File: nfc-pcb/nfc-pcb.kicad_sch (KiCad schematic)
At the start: 1 part, among them U1 NT3H1101W0FHKH

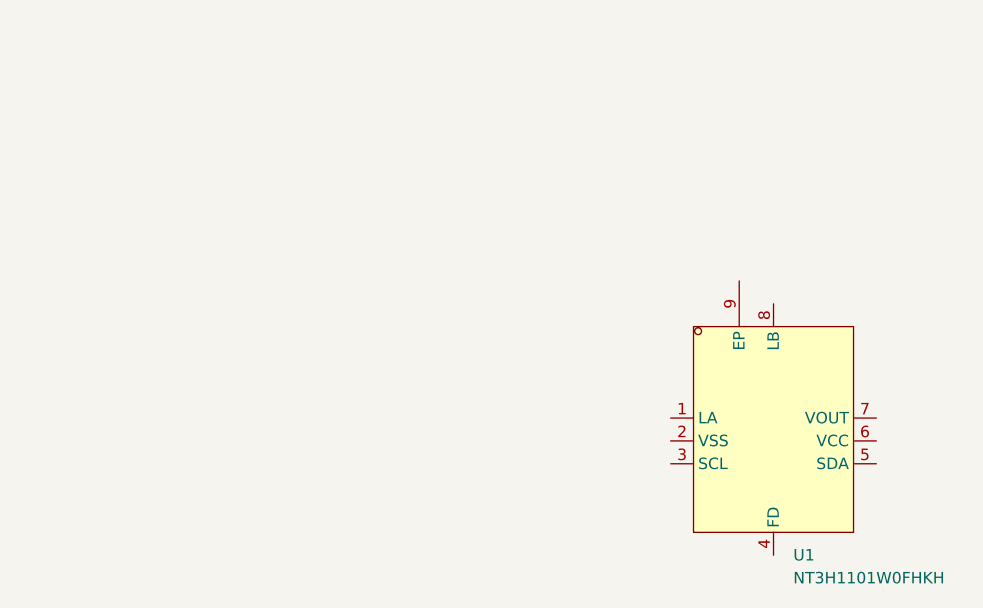
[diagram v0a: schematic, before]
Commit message: update
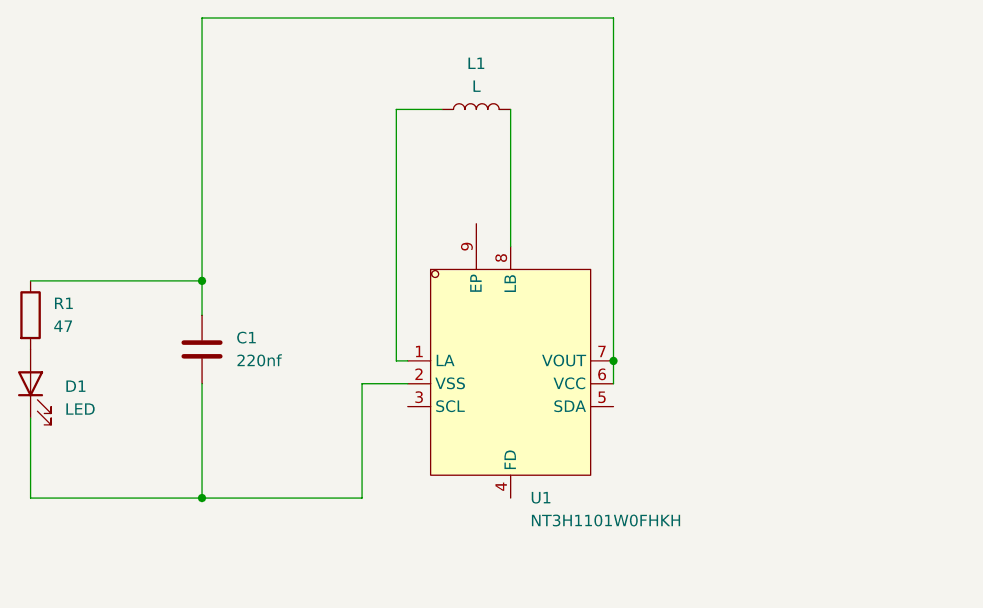
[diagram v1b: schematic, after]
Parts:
- added C1: 220nf, symbol Device:C
- added D1: LED, symbol Device:LED
- added L1: L, symbol Device:L
- added R1: 47, symbol Device:R
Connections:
- net at U1.1 (LA): now also L1.1
- net at U1.2 (VSS): now also C1.2, D1.1 (K)
- net at U1.6 (VCC): now also U1.7 (VOUT), C1.1, R1.1
- net at U1.8 (LB): now also L1.2
- new net: D1.2 (A), R1.2
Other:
- moved on the sheet: U1

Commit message: update
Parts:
- C1: footprint (none) -> Capacitor_SMD:C_1206_3216Metric
- D1: footprint (none) -> LED_SMD:LED_1206_3216Metric
- L1: footprint (none) -> nfc_ant:antenna-nfc
- R1: footprint (none) -> Resistor_SMD:R_1206_3216Metric
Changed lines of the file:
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@@
 			)
 		)
-		(property "Footprint" ""
+		(property "Footprint" "Capacitor_SMD:C_1206_3216Metric"
 			(at 186.3852 64.77 0)
 			(effects
@@
 			)
 		)
-		(property "Footprint" ""
+		(property "Footprint" "nfc_ant:antenna-nfc"
 			(at 215.9 34.29 0)
 			(effects
@@
 			)
 		)
-		(property "Footprint" ""
+		(property "Footprint" "Resistor_SMD:R_1206_3216Metric"
 			(at 164.592 57.15 90)
 			(effects
@@
 			)
 		)
-		(property "Footprint" ""
+		(property "Footprint" "LED_SMD:LED_1206_3216Metric"
 			(at 166.37 64.77 0)
 			(effects
